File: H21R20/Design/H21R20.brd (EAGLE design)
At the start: 34.6 x 30 mm, 54 parts, among them IC1 ESP32-C3-MINI-1-N4, P1 HEXABIT_17.32_NO_P6_P7_P12, Q1 MMBT3904LT1, U1 STM32G0B1CEU6NUFQFPN48_STM32_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, X1 XTALL_CSTCE8M00G52

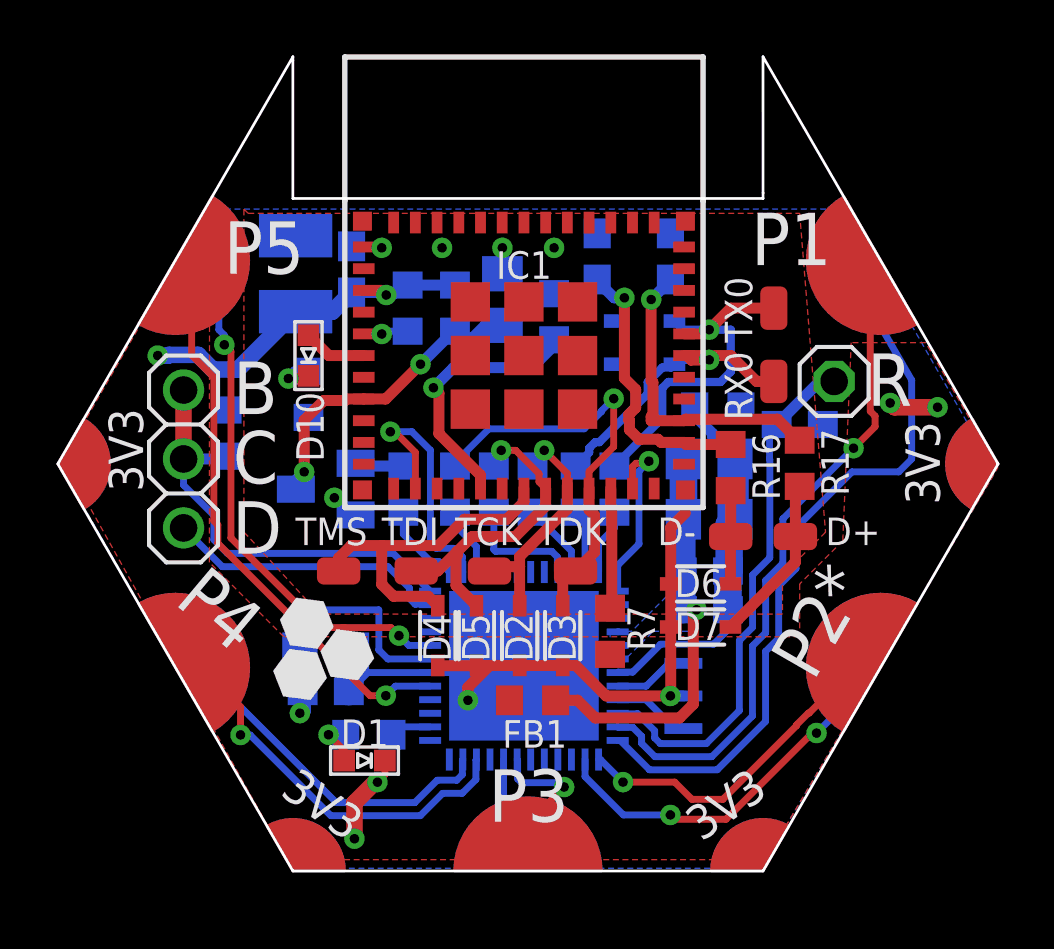
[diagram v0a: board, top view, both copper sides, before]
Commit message: -Changing some issues in the design to improve the performance
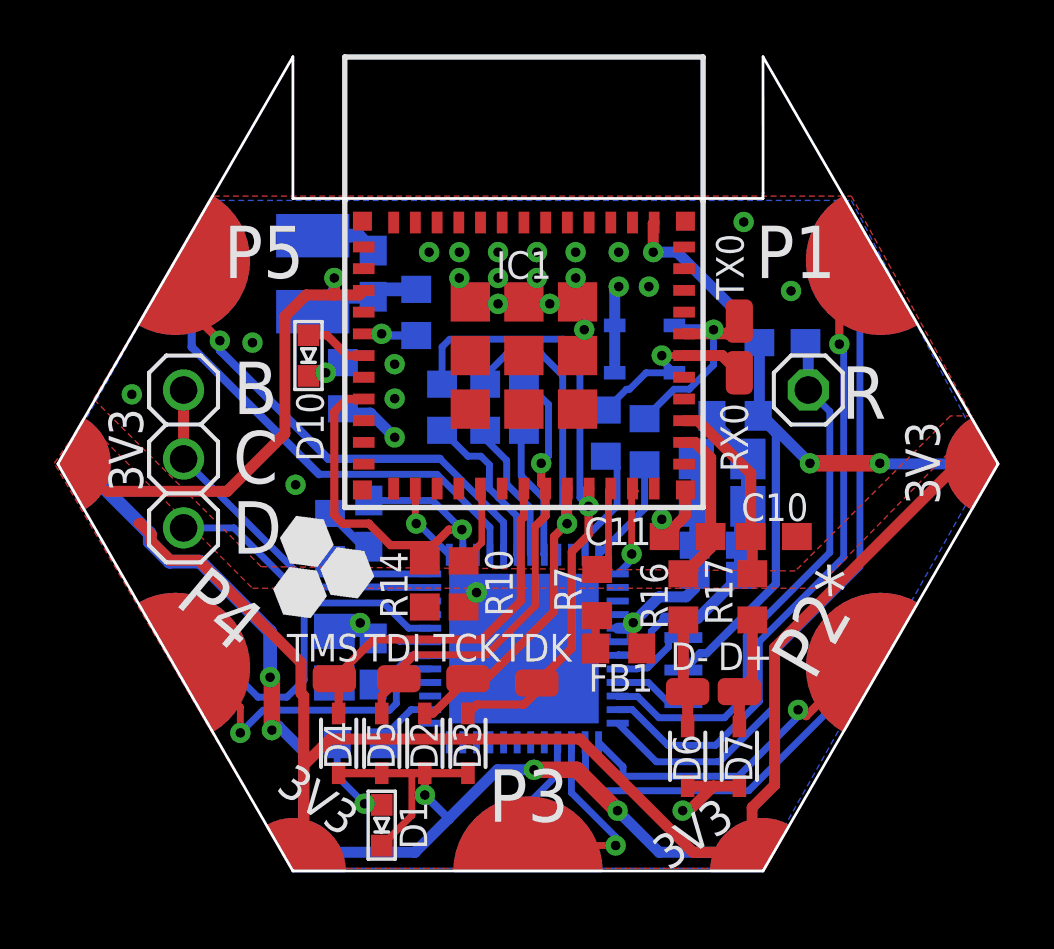
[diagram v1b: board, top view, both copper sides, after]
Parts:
- removed C9: 1uF, HEXABITZ_RCLS:C-0805-POL
- removed Q1: MMBT3904LT1, HEXABITZ_RCLS:MMBT3904LT1
- removed R15: 10K, HEXABITZ_RCLS:R-0603
- added C2: 100nF, HEXABITZ_RCLS:C-0603
- X1: value XTALL_CSTCE8M00G52 -> 8MHZ
- moved C10 11.0 mm to (44.0, 31.4), flipped to the top, turned to 180 degrees
- moved C11 10.8 mm to (40.8, 31.4), flipped to the top, turned to 0 degrees
- moved R10 10.4 mm to (32.5, 29.7), flipped to the top, turned to 270 degrees
- moved R14 10.2 mm to (31.1, 29.7), flipped to the top, turned to 90 degrees
- moved D6 6.37 mm to (40.8, 23.3), turned to 90 degrees
- moved D+ 6.08 mm to (42.7, 25.7)
- moved D- 5.93 mm to (40.8, 25.7)
- moved D4 5.39 mm to (27.9, 23.8)
- moved R2 5.39 mm to (27.6, 31.4)
- moved D2 5.29 mm to (31.1, 23.8)
- moved D5 5.29 mm to (29.5, 23.8)
- moved D3 5.29 mm to (32.7, 23.8)
- moved R17 5.22 mm to (43.2, 29.2)
- moved R16 5.07 mm to (40.6, 29.2)
- moved D7 4.97 mm to (42.7, 23.3), turned to 90 degrees
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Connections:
- removed net N$11 (its old number): D5.2, IC1.19, R13.1, TDI.P$1
- removed net N$13: Q1.1, R15.2
- removed net N$25: C9.1, IC1.8, Q1.3, R14.2
- removed net N$8: D2.2, IC1.20, R12.1, TCK.P$1
- removed net USART3_RX: P1.PAD_PD4, U1.23
- removed net USART3_TX: P1.PAD_PU4, U1.22
- new net N$10: D2.2, IC1.20, R13.1, TCK.P$1
- new net N$18: D5.2, IC1.19, R12.1, TDI.P$1
- new net USART6_RX: P1.PAD_PD3, U1.16
- new net USART6_TX: P1.PAD_PU3, U1.15
- net ESP32_CS: now also U1.37; no longer U1.38
- net ESP32_MISO: now also U1.43; no longer U1.45
- net ESP32_MOSI: now also U1.44; no longer U1.46
- net ESP32_RESET: now also C2.2, IC1.8, R14.2, U1.38; no longer R15.1, U1.37
- net ESP32_SCK: now also U1.42; no longer U1.39
- net GND: now also C2.1, U1.2, U1.23, U1.3; no longer C9.2, Q1.2
- net N$6: now also D9.2; no longer D8.2
- net N$7: now also D8.2; no longer D9.2
- net USART1_RX: now also P1.PAD_PD4; no longer P1.PAD_PD5
- net USART1_TX: now also P1.PAD_PU4; no longer P1.PAD_PU5
- net USART5_RX: now also P1.PAD_PD5, U1.40; no longer P1.PAD_PD3, U1.20
- net USART5_TX: now also P1.PAD_PU5, U1.41; no longer P1.PAD_PU3, U1.19
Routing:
- net GND: track 31.8 -> 99.9 mm, vias 11 -> 34
- net VDD: track 25.2 -> 79.1 mm, vias 3 -> 2
- net N$10: track 0.00 -> 20.4 mm, vias 0 -> 1
- net N$18: track 0.00 -> 17.1 mm, vias 0 -> 1
- net USART3_TX: track 14.8 -> 0.00 mm, vias 1 -> 0
- net USART5_RX: track 3.79 -> 17.6 mm
- net USART3_RX: track 13.2 -> 0.00 mm
- net ESP32_RESET: track 3.08 -> 15.9 mm, vias 0 -> 1
- net USART5_TX: track 5.52 -> 17.7 mm
- net N$11 (its old number): track 11.8 -> 0.00 mm, vias 1 -> 0
- net N$25: track 11.8 -> 0.00 mm, vias 2 -> 0
- net N$8: track 9.02 -> 0.00 mm, vias 1 -> 0
- net USART1_TX: track 20.8 -> 11.8 mm
- net N$11: track 15.6 -> 23.7 mm
- net USART6_TX: track 0.00 -> 7.81 mm, vias 0 -> 1
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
